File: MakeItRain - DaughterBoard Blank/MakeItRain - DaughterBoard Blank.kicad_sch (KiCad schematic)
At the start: 1 part, among them J1 Conn_02x15_Odd_Even

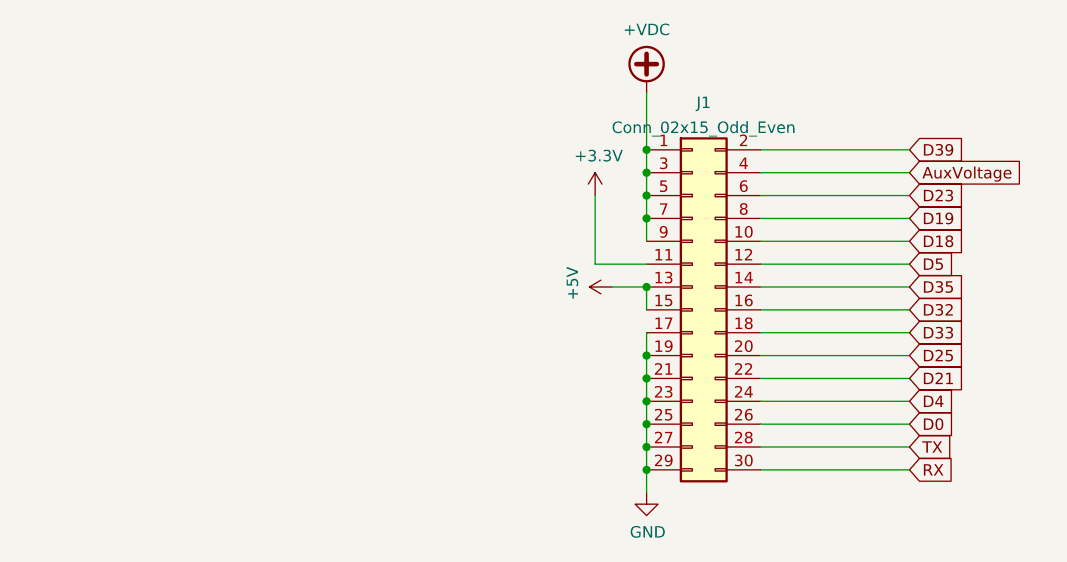
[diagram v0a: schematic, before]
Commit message: updating some routes, updating the already done daughterboard and updating the blank layout for both.
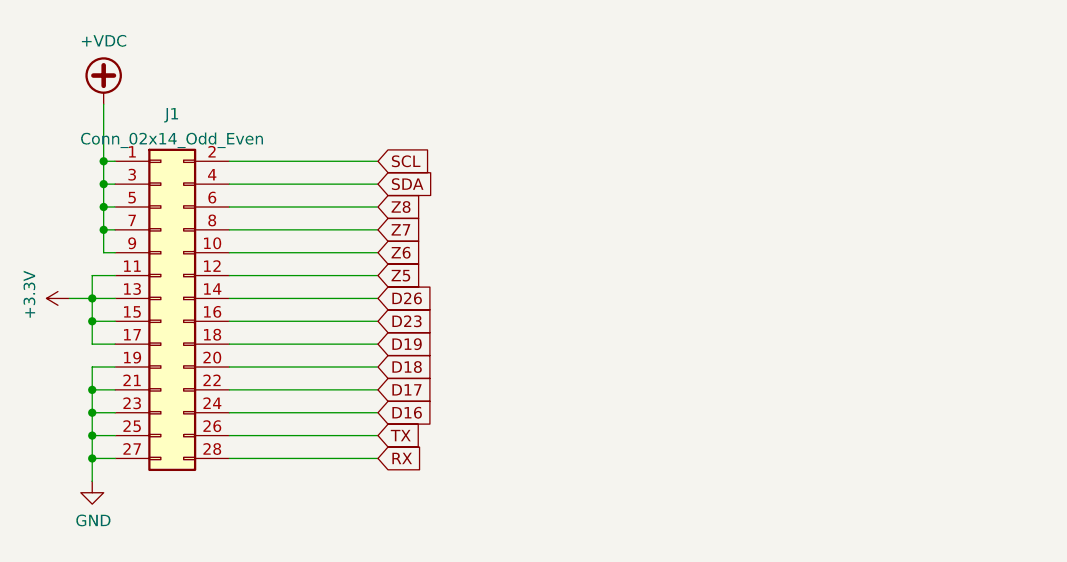
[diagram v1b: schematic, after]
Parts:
- removed J1: Conn_02x15_Odd_Even, Connector_PinHeader_2.54mm:PinHeader_2x15_P2.54mm_Vertical, symbol Connector_Generic:Conn_02x15_Odd_Even
- added J1: Conn_02x14_Odd_Even, Connector_PinHeader_2.54mm:PinHeader_2x14_P2.54mm_Vertical, symbol Connector_Generic:Conn_02x14_Odd_Even
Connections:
- net +3V3: now also J1.11 (Pin_11), J1.13 (Pin_13), J1.15 (Pin_15), J1.17 (Pin_17)
- net +VDC: now also J1.1 (Pin_1), J1.3 (Pin_3), J1.5 (Pin_5), J1.7 (Pin_7), J1.9 (Pin_9)
- net D18: now also J1.20 (Pin_20)
- net D19: now also J1.18 (Pin_18)
- net D23: now also J1.16 (Pin_16)
- net GND: now also J1.19 (Pin_19), J1.21 (Pin_21), J1.23 (Pin_23), J1.25 (Pin_25), J1.27 (Pin_27)
- net RX: now also J1.28 (Pin_28)
- net TX: now also J1.26 (Pin_26)
- new net D16: J1.24 (Pin_24)
- new net D17: J1.22 (Pin_22)
- new net D26: J1.14 (Pin_14)
- new net SCL: J1.2 (Pin_2)
- new net SDA: J1.4 (Pin_4)
- new net Z5: J1.12 (Pin_12)
- new net Z6: J1.10 (Pin_10)
- new net Z7: J1.8 (Pin_8)
- new net Z8: J1.6 (Pin_6)
